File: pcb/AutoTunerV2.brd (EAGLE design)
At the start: 100 x 90 mm, 80 parts, among them IC1 TP4054-42-SOT25-R, IC2 317EMP, IC4 LM324_SOIC, Q1 32,768kHz, Q2 BSS123, Q3 BSS84, U1 STM32F103C8T6, U2 TPS613222ADBVR, Y1 8MHz

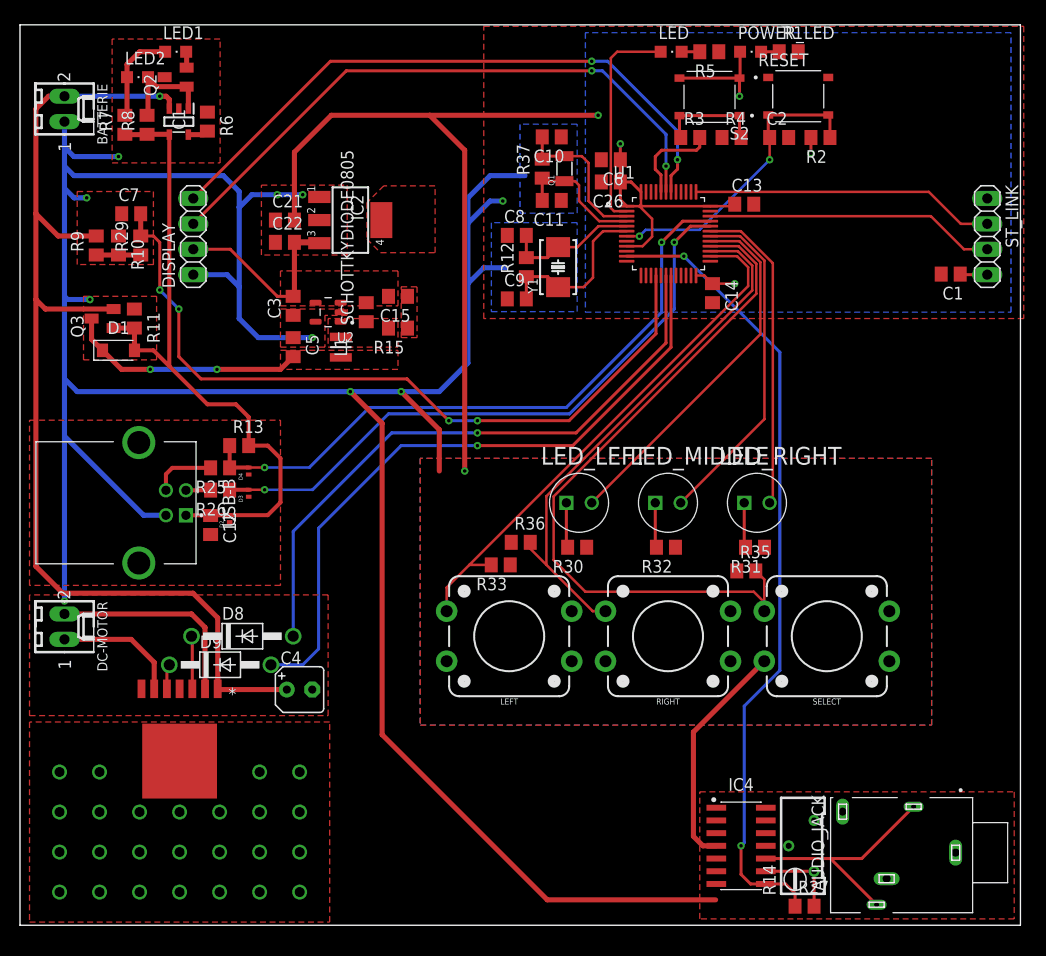
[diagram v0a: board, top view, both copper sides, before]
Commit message: board v2 release 2.0
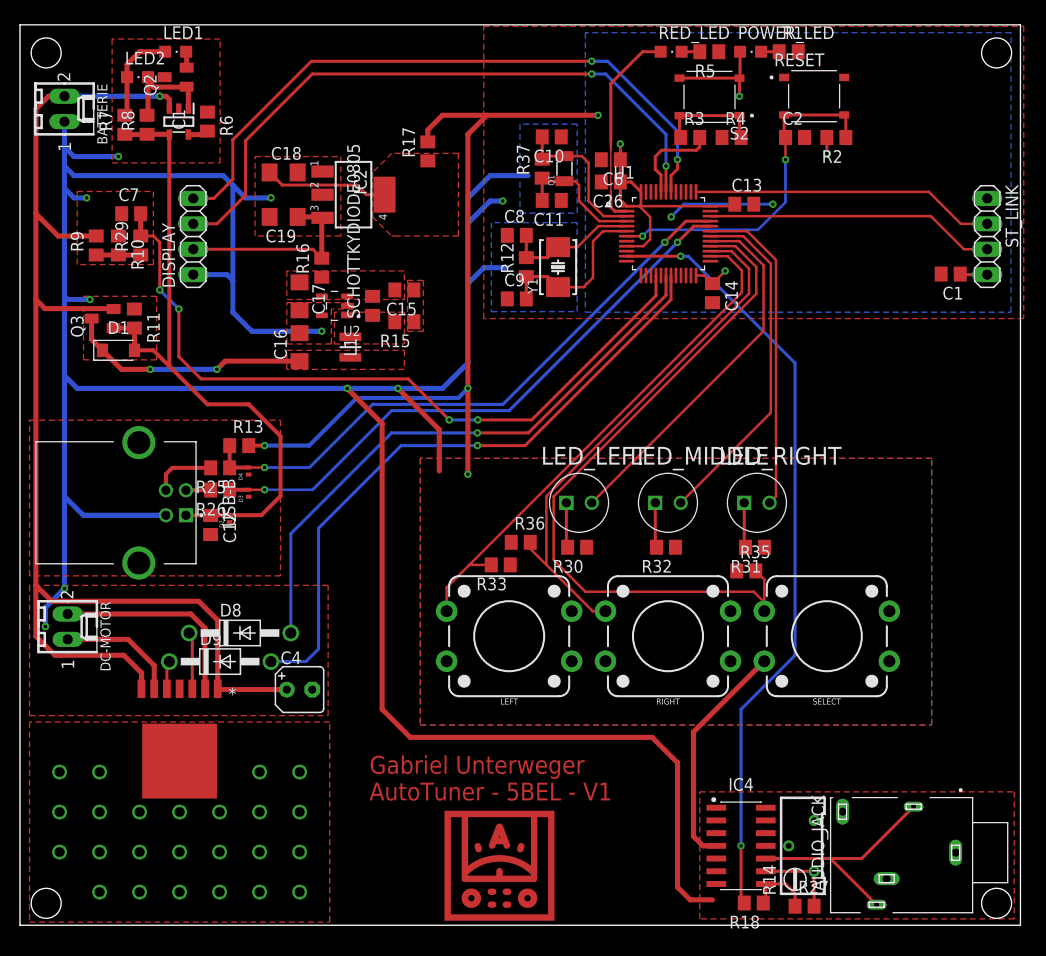
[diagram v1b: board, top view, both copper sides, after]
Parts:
- removed C21, C22: (no value), rcl:C0805
- removed C3, C5: 22u, rcl:C0805
- added C16, C17, C18, C19: 22u, rcl:C1206
- added R16, R17, R18: 0, rcl:R0805
- R1, R5: value 500 -> 68
- R13: value 1k5 / 4k7 -> 1k5
- R15: value 5 -> 5R
- R30, R31, R32: value (none) -> 100
- moved IC2 2.56 mm to (33.3, 73.0)
- moved C2 1.59 mm to (77.5, 78.7)
- moved RESET 1.59 mm to (79.4, 82.9)
- moved R2 1.59 mm to (81.6, 78.7)
- moved L1 0.95 mm to (33.0, 57.8)
- moved R15 0.90 mm to (38.4, 60.3)
- moved U2 0.90 mm to (31.4, 61.9)
- moved C15 0.90 mm to (38.4, 63.5)
- moved SCHOTTKYDIODE0805 0.90 mm to (35.2, 61.9)
- moved D8 0.40 mm to (22.0, 29.2)
- moved DC-MOTOR 0.32 mm to (4.76, 29.8)
- moved D9 0.32 mm to (20.0, 26.4)
- renumbered LED to RED_LED
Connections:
- new net N$13: C18.1, IC2.4, R17.1
- new net N$45: R18.2, U1.11
- net +3V3: now also R13.2, R17.2; no longer C21.2, IC2.4
- net +5V: now also C19.1, R16.2; no longer C15.2, C22.2, C3.2, SCHOTTKYDIODE0805.2, U2.4
- net GND: now also C16.2, C17.2, C18.2, C19.2; no longer C21.1, C22.1, C3.1, C5.1
- net N$7: now also C15.2, C17.1, R16.1, SCHOTTKYDIODE0805.2, U2.4; no longer U4.7
- net SIGNAL_OPAMP: now also R18.1; no longer U1.11
- net VBAT: now also U4.7
- net VBUS: no longer R13.2
- net VIN: now also C16.1; no longer C5.2
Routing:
- net N$45: track 0.00 -> 77.6 mm, vias 0 -> 2
- net SIGNAL_OPAMP: track 80.6 -> 6.60 mm, vias 2 -> 0
- net VBAT: track 110.1 -> 129.8 mm
- net GND: track 283.0 -> 298.4 mm, vias 10 -> 12
- net N$13: track 0.00 -> 12.4 mm, vias 1 -> 0
- net USB+: track 64.6 -> 60.5 mm
- net RESET: track 30.3 -> 34.4 mm
- net USB-: track 62.9 -> 59.0 mm
- net +3V3: track 145.6 -> 149.2 mm, vias 6 -> 8
- net MOTOR_PWM1: track 62.3 -> 59.3 mm
- net DISPLAY_SDA: track 62.0 -> 64.9 mm
- net MOTOR_PWM2: track 67.4 -> 64.5 mm
- net DISPLAY_SCL: track 63.3 -> 65.6 mm
- net BATTERY_LEVEL: track 76.4 -> 74.1 mm
- net PC13: track 21.9 -> 20.4 mm
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- added copper zone on layer 1, net N$13
- added copper zone on layer 1, net N$7
- removed copper zone on layer 1, net +3V3
- removed copper zone on layer 1, net +5V
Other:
- board text added: "Gabriel Unterweger AutoTuner - 5BEL - V1"

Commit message: board v2 main release & oder
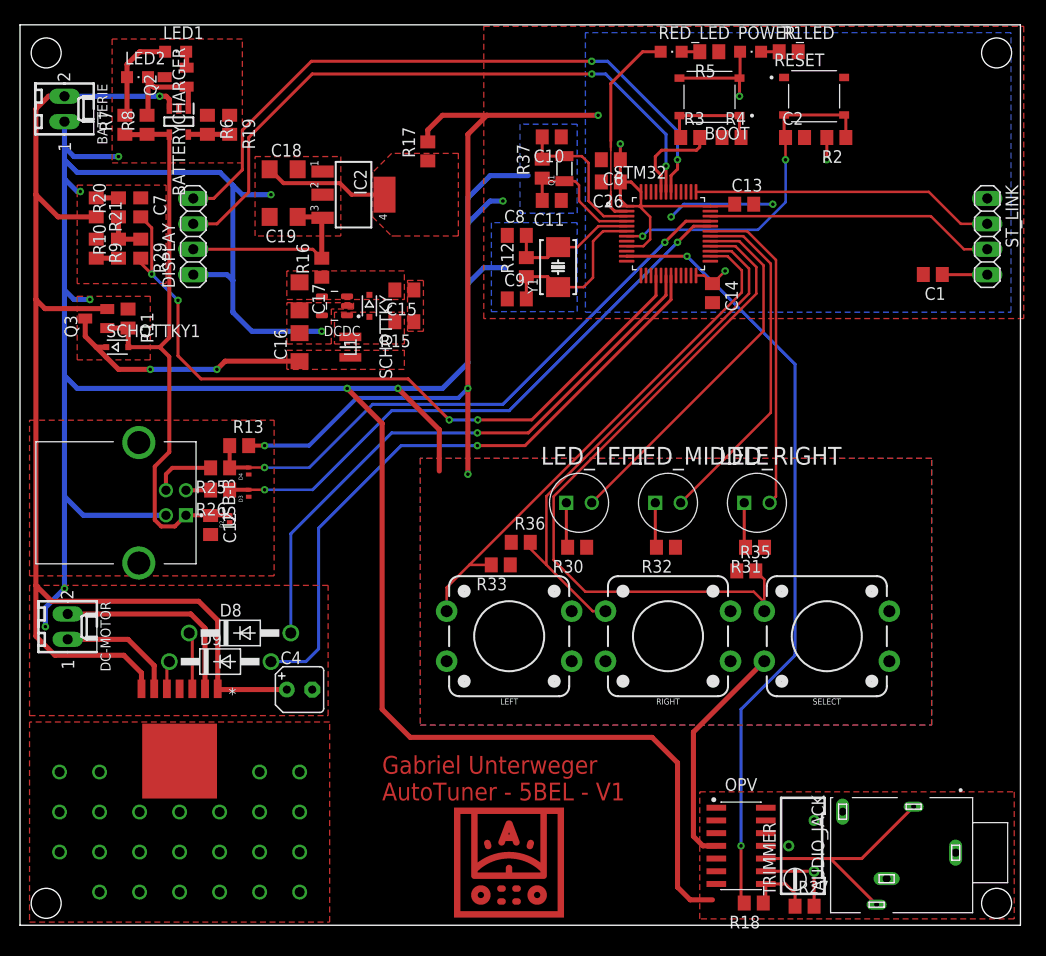
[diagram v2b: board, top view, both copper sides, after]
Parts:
- removed D1: MBR0520LT1G, Diode:SODFL3718X115
- removed SCHOTTKYDIODE0805: (no value), rcl:C0805
- added R19: 6k8, rcl:R0805
- added R20: 330k, rcl:R0805
- added R21: 470k, rcl:R0805
- added SCHOTTKY, SCHOTTKY1: (no value), diode:SOD323-R
- BOOT: value TS-1187A-B-A-B -> (none)
- C4: value 10-100uF -> 100uF
- OPV: value LM324_SOIC -> (none)
- R10: value 2M -> 1M
- R6: value 1k66 -> 2k2
- R9: value 800k -> 1M
- moved C1 1.79 mm to (91.2, 65.0)
- moved C7 1.14 mm to (12.1, 71.8), turned to 270 degrees
- moved Q3 0.64 mm to (7.62, 60.6)
- moved R11 0.63 mm to (10.8, 60.6)
- moved C18 0.32 mm to (26.4, 75.6)
- moved R10 0.32 mm to (9.84, 67.6), turned to 90 degrees
- moved R29 0.32 mm to (12.1, 67.6), turned to 270 degrees
- moved R6 0.32 mm to (18.7, 80.0)
- moved R9 0.32 mm to (7.62, 67.6), turned to 270 degrees
- renumbered IC1 to BATTERYCHARGER, IC4 to OPV, R14 to TRIMMER, S2 to BOOT, U1 to STM32, U2 to DCDC, U4 to H-BRUECKE
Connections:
- new net N$46: R20.2, R21.1
- new net N$47: R10.2, R20.1, R29.1
- net GND: now also R19.1, R9.1; no longer R10.1
- net N$1: now also SCHOTTKY.A; no longer SCHOTTKYDIODE0805.1
- net N$4: now also R10.1, R9.2; no longer R10.2, R29.1, R9.1
- net N$7: now also SCHOTTKY.C; no longer SCHOTTKYDIODE0805.2
- net N$8: now also R19.2
- net VBAT: now also R21.2; no longer R9.2
- net VBUS: now also SCHOTTKY1.A; no longer D1.2
- net VIN: now also SCHOTTKY1.C; no longer D1.1
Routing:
- net VBUS: track 66.4 -> 59.8 mm
- net N$47: track 0.00 -> 4.45 mm
- net +3V3: track 149.2 -> 151.6 mm
- net N$4: track 4.44 -> 2.22 mm
- net N$46: track 0.00 -> 2.22 mm
- net N$8: track 2.05 -> 4.14 mm
- net VIN: track 24.5 -> 25.9 mm
- net BATTERY_LEVEL: track 74.1 -> 75.1 mm
- net VBAT: track 129.8 -> 129.2 mm
